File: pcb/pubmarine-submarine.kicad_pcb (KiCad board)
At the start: 2 copper layers, 150.5 x 100 mm, 68 parts, among them J1 GPIO_IN, J10 RPD, J11 Screw_Terminal_01x08, J12 Screw_Terminal_01x08, J13 ADC_HDR, J14 PWM_HDR, J2 GPIO_OUT, J3 FYL, J4 FYR, J5 FPU, J6 FPD, J7 RPU, J8 RYL, J9 RYR, Q1 AO3400A, Q2 AO3400A, Q3 AO3400A, Q4 AO3400A, Q5 AO3400A, Q6 AO3400A, Q7 AO3400A, Q8 AO3400A, U1 A4950E, U2 A4950E, U3 A4950E, U4 A4950E, U5 TLC5947DAP, U6 MCP3008

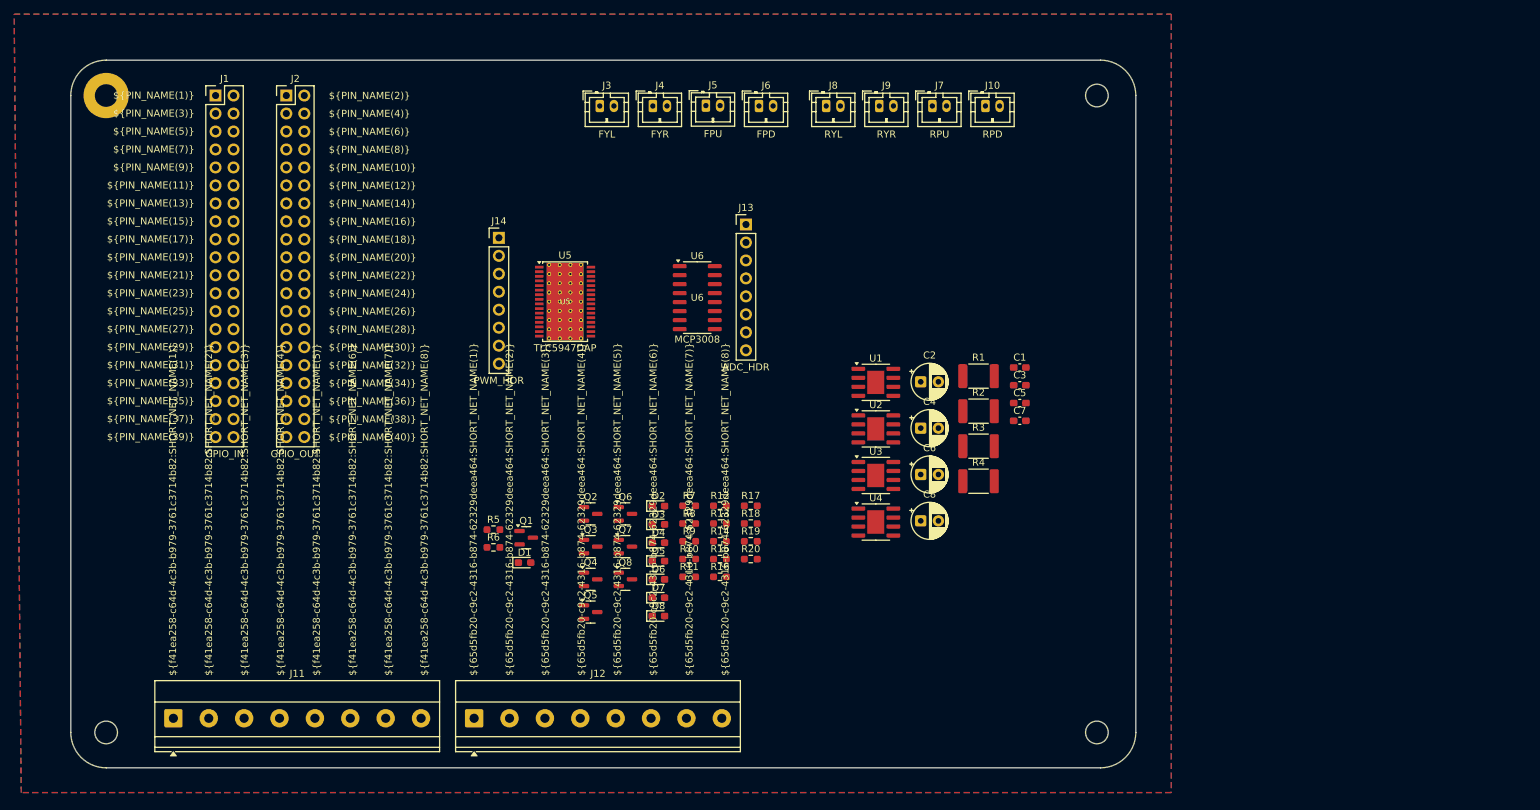
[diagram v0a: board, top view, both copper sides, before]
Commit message: new PCB
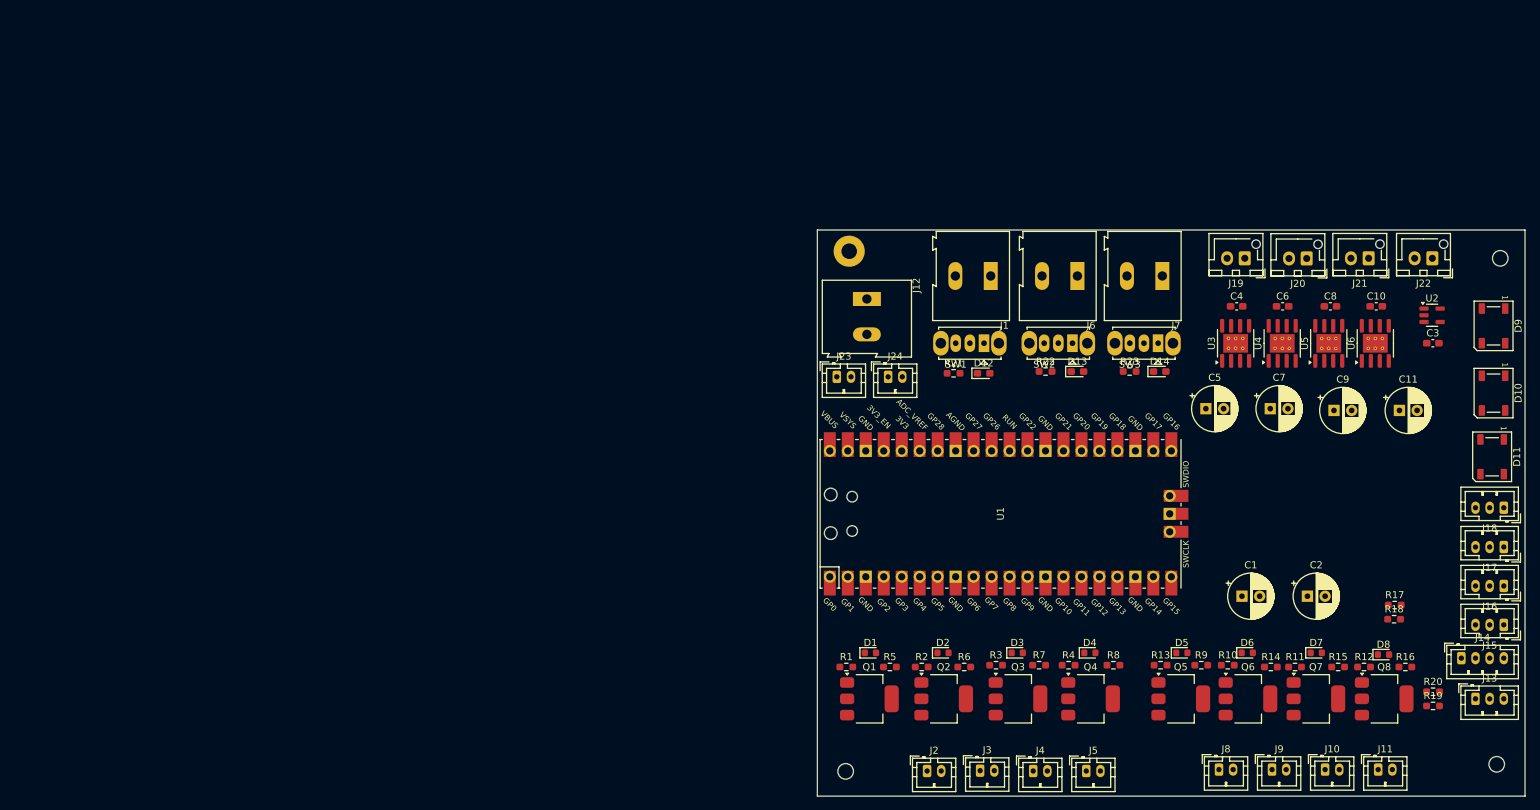
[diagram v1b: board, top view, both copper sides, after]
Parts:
- added C10: 0.22uF, Capacitor_SMD:C_0603_1608Metric_Pad1.08x0.95mm_HandSolder, F.Cu at (254.5, 69.8)
- added C11: 100uF, Capacitor_THT:CP_Radial_D6.3mm_P2.50mm, F.Cu at (257.8, 84.5)
- added C9: 100uF, Capacitor_THT:CP_Radial_D6.3mm_P2.50mm, F.Cu at (248.5, 84.5)
- added D10: WS2812B, LED_SMD:LED_WS2812B_PLCC4_5.0x5.0mm_P3.2mm, F.Cu at (271.1, 82.0)
- added D11: WS2812B, LED_SMD:LED_WS2812B_PLCC4_5.0x5.0mm_P3.2mm, F.Cu at (270.9, 91.0)
- added D12: LED, LED_SMD:LED_0603_1608Metric_Pad1.05x0.95mm_HandSolder, F.Cu at (199.0, 79.2)
- added D13: LED, LED_SMD:LED_0603_1608Metric_Pad1.05x0.95mm_HandSolder, F.Cu at (212.2, 79.0)
- added D14: LED, LED_SMD:LED_0603_1608Metric_Pad1.05x0.95mm_HandSolder, F.Cu at (223.9, 79.0)
- added D9: WS2812B, LED_SMD:LED_WS2812B_PLCC4_5.0x5.0mm_P3.2mm, F.Cu at (271.1, 72.5)
- added J15: Servo1, Connector_JST:JST_PH_B3B-PH-K_1x03_P2.00mm_Vertical, F.Cu at (272.5, 114.8)
- added J16: Servo2, Connector_JST:JST_PH_B3B-PH-K_1x03_P2.00mm_Vertical, F.Cu at (272.5, 109.3)
- added J17: Servo3, Connector_JST:JST_PH_B3B-PH-K_1x03_P2.00mm_Vertical, F.Cu at (272.5, 103.8)
- added J18: Servo4, Connector_JST:JST_PH_B3B-PH-K_1x03_P2.00mm_Vertical, F.Cu at (272.5, 98.2)
- added J19: Conn_01x02, Connector_JST:JST_XH_B2B-XH-AM_1x02_P2.50mm_Vertical, F.Cu at (235.9, 63.0)
- added J20: Conn_01x02, Connector_JST:JST_XH_B2B-XH-AM_1x02_P2.50mm_Vertical, F.Cu at (244.7, 63.0)
- added J21: Conn_01x02, Connector_JST:JST_XH_B2B-XH-AM_1x02_P2.50mm_Vertical, F.Cu at (253.4, 63.0)
- added J22: Conn_01x02, Connector_JST:JST_XH_B2B-XH-AM_1x02_P2.50mm_Vertical, F.Cu at (262.4, 63.0)
- added J23: Conn_01x02, Connector_JST:JST_PH_B2B-PH-K_1x02_P2.00mm_Vertical, F.Cu at (178.2, 79.8)
- added J24: Conn_01x02, Connector_JST:JST_PH_B2B-PH-K_1x02_P2.00mm_Vertical, F.Cu at (185.5, 79.8)
- added R21: 1K, Resistor_SMD:R_0603_1608Metric_Pad0.98x0.95mm_HandSolder, F.Cu at (194.8, 79.2)
- added R22: 330, Resistor_SMD:R_0603_1608Metric_Pad0.98x0.95mm_HandSolder, F.Cu at (207.8, 79.0)
- added R23: 330, Resistor_SMD:R_0603_1608Metric_Pad0.98x0.95mm_HandSolder, F.Cu at (219.6, 79.0)
- added SW1: SW_SPDT, Button_Switch_THT:SW_Slide_SPDT_Straight_CK_OS102011MS2Q, F.Cu at (199.1, 75.0)
- added SW2: SW_SPDT, Button_Switch_THT:SW_Slide_SPDT_Straight_CK_OS102011MS2Q, F.Cu at (211.6, 75.0)
- added SW3: SW_SPDT, Button_Switch_THT:SW_Slide_SPDT_Straight_CK_OS102011MS2Q, F.Cu at (223.7, 75.0)
- C1, C5, C7: value 0.22uF -> 100uF; footprint Capacitor_SMD:C_0603_1608Metric_Pad1.08x0.95mm_HandSolder -> Capacitor_THT:CP_Radial_D6.3mm_P2.50mm
- C2: footprint Capacitor_THT:CP_Radial_D5.0mm_P2.50mm -> Capacitor_THT:CP_Radial_D6.3mm_P2.50mm
- C3: value 0.22uF -> 0.1uF
- C4, C6, C8: value 100uF -> 0.22uF; footprint Capacitor_THT:CP_Radial_D5.0mm_P2.50mm -> Capacitor_SMD:C_0603_1608Metric_Pad1.08x0.95mm_HandSolder
- D1, D2, D3, D4, D5, D6, D7, D8: value D_Schottky -> 1N5822; footprint Diode_SMD:D_0603_1608Metric_Pad1.05x0.95mm_HandSolder -> Diode_SMD:D_0603_1608Metric
- H1: value MountingHole_Pad -> MountingHole; footprint MountingHole:MountingHole_3.2mm_M3_Pad -> MountingHole:MountingHole_2.2mm_M2
- H2, H3: footprint MountingHole:MountingHole_3.2mm_M3 -> MountingHole:MountingHole_2.2mm_M2
- H4: value MountingHole -> MountingHole_Pad; footprint MountingHole:MountingHole_3.2mm_M3 -> MountingHole:MountingHole_2.2mm_M2_Pad
- J1: value GPIO_IN -> Screw_Terminal_01x02; footprint Connector_PinHeader_2.54mm:PinHeader_2x20_P2.54mm_Vertical -> TerminalBlock:TerminalBlock_Altech_AK300-2_P5.00mm
- J10: value RPD -> Conn_01x02
- J11: value Screw_Terminal_01x08 -> Conn_01x02; footprint TerminalBlock_Phoenix:TerminalBlock_Phoenix_MKDS-1,5-8_1x08_P5.00mm_Horizontal -> Connector_JST:JST_PH_B2B-PH-K_1x02_P2.00mm_Vertical
- J12: value Screw_Terminal_01x08 -> Screw_Terminal_01x02; footprint TerminalBlock_Phoenix:TerminalBlock_Phoenix_MKDS-1,5-8_1x08_P5.00mm_Horizontal -> TerminalBlock:TerminalBlock_Altech_AK300-2_P5.00mm
- J13: value ADC_HDR -> Conn_01x03; footprint Connector_PinHeader_2.54mm:PinHeader_1x08_P2.54mm_Vertical -> Connector_JST:JST_PH_B3B-PH-K_1x03_P2.00mm_Vertical
- J14: value PWM_HDR -> Conn_01x04; footprint Connector_PinHeader_2.54mm:PinHeader_1x08_P2.54mm_Vertical -> Connector_JST:JST_PH_B4B-PH-K_1x04_P2.00mm_Vertical
- J2: value GPIO_OUT -> Conn_01x02; footprint Connector_PinHeader_2.54mm:PinHeader_2x20_P2.54mm_Vertical -> Connector_JST:JST_PH_B2B-PH-K_1x02_P2.00mm_Vertical
- J3: value FYL -> Conn_01x02
- J4: value FYR -> Conn_01x02
- J5: value FPU -> Conn_01x02
- J6: value FPD -> Screw_Terminal_01x02; footprint Connector_JST:JST_PH_B2B-PH-K_1x02_P2.00mm_Vertical -> TerminalBlock:TerminalBlock_Altech_AK300-2_P5.00mm
- J7: value RPU -> Screw_Terminal_01x02; footprint Connector_JST:JST_PH_B2B-PH-K_1x02_P2.00mm_Vertical -> TerminalBlock:TerminalBlock_Altech_AK300-2_P5.00mm
- J8: value RYL -> Conn_01x02
- J9: value RYR -> Conn_01x02
- Q1, Q2, Q3, Q4, Q5, Q6, Q7, Q8: value AO3400A -> Q_NMOS_Depletion_DGS; footprint Package_TO_SOT_SMD:SOT-23 -> Package_TO_SOT_SMD:SOT-223-3_TabPin2
- R1, R2, R3, R4: value 1.1Ω -> 470; footprint Resistor_SMD:R_1812_4532Metric_Pad1.30x3.40mm_HandSolder -> Resistor_SMD:R_0603_1608Metric_Pad0.98x0.95mm_HandSolder
- R10, R12: value 100 -> 470
- R11, R9: value 1K -> 470
- R13, R15, R6, R7: value 1K -> 10k
- R14, R16, R5, R8: value 100 -> 10k
- R17: value 1K -> 4.7K
- R18: value 100 -> 4.7K
- R19: value 1K -> 10K
- R20: value 100 -> 20K
- U1: value A4950E -> Pico; footprint Package_SO:SOIC-8-1EP_3.9x4.9mm_P1.27mm_EP2.41x3.3mm -> MCU_RaspberryPi_and_Boards:RPi_Pico_SMD_TH
- U2: value A4950E -> SN74LV1T34DBV; footprint Package_SO:SOIC-8-1EP_3.9x4.9mm_P1.27mm_EP2.41x3.3mm -> Package_TO_SOT_SMD:SOT-23-5
- U3, U4: footprint Package_SO:SOIC-8-1EP_3.9x4.9mm_P1.27mm_EP2.41x3.3mm -> Package_SO:SOIC-8-1EP_3.9x4.9mm_P1.27mm_EP2.62x3.51mm_ThermalVias
- U5: value TLC5947DAP -> A4950E; footprint Package_SO:HTSSOP-32-1EP_6.1x11mm_P0.65mm_EP5.2x11mm_Mask4.11x4.36mm_ThermalVias -> Package_SO:SOIC-8-1EP_3.9x4.9mm_P1.27mm_EP2.62x3.51mm_ThermalVias
- U6: value MCP3008 -> A4950E; footprint Package_SO:SOIC-16_3.9x9.9mm_P1.27mm -> Package_SO:SOIC-8-1EP_3.9x4.9mm_P1.27mm_EP2.62x3.51mm_ThermalVias
- moved H1 198.3 mm to (272.0, 63.0)
- moved J11 170.4 mm to (254.8, 135.2)
- moved J14 148.4 mm to (266.5, 119.5)
- moved J2 131.6 mm to (191.0, 135.4)
- moved J13 123.0 mm to (268.5, 125.2)
- moved J1 112.5 mm to (200.0, 65.5), turned to 180 degrees
- moved H2 110.1 mm to (271.5, 134.5)
- moved J8 109.0 mm to (232.2, 135.2)
- moved J9 109.0 mm to (239.8, 135.2)
- moved Q8 108.6 mm to (255.6, 125.2)
- moved J5 108.3 mm to (213.5, 135.4)
- moved J4 108.3 mm to (206.0, 135.4)
- moved J3 108.2 mm to (198.5, 135.4)
- moved U5 108.1 mm to (247.8, 75.0), turned to 90 degrees
- moved J10 105.3 mm to (247.2, 135.2)
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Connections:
- C1 pad 1: +12VA -> +5VP
- C1 pad 2: GNDA -> GND
- C2 pad 1: +12VA -> +5VP
- C2 pad 2: GNDA -> GND
- C3 pad 1: +12VA -> +5VL
- C3 pad 2: GNDA -> GND
- C4 pad 1: +12VA -> +12V
- C4 pad 2: GNDA -> GND
- C5 pad 1: +12VA -> +12V
- C5 pad 2: GNDA -> GND
- C6 pad 1: +12VA -> +12V
- C6 pad 2: GNDA -> GND
- C7 pad 1: +12VA -> +12V
- C7 pad 2: GNDA -> GND
- C8 pad 1: +12VA -> +12V
- C8 pad 2: GNDA -> GND
- D1 pad 1: +12VA -> +5VP
- D1 pad 2: FYL- -> /FU-
- D2 pad 1: +12VA -> +5VP
- D2 pad 2: FYR- -> /FD-
- D3 pad 1: +12VA -> +5VP
- D3 pad 2: FPU- -> /FL-
- D4 pad 1: +12VA -> +5VP
- D4 pad 2: FPD- -> /FR-
- D5 pad 1: +12VA -> +5VP
- D5 pad 2: RYL- -> /RU-
- D6 pad 1: +12VA -> +5VP
- D6 pad 2: RYR- -> /RD-
- D7 pad 1: +12VA -> +5VP
- D7 pad 2: RPU- -> /RL-
- D8 pad 1: +12VA -> +5VP
- D8 pad 2: RPD- -> /RR-
- J1 pad 1: unconnected-(J1-3V3-Pad1) -> Net-(J1-Pin_1)
- J1 pad 2: +5VD -> GND
- J10 pad 1: +12VA -> +5VP
- J10 pad 2: RPD- -> /RL-
- J11 pad 1: +12VA -> +5VP
- J11 pad 2: GNDA -> /RR-
- J12 pad 1: X+ -> +5VL
- J12 pad 2: X- -> GND
- J13 pad 1: CH0 -> GND
- J13 pad 2: CH1 -> +5VL
- J13 pad 3: CH2 -> Net-(J13-Pin_3)
- J14 pad 1: PWM16 -> GND
- J14 pad 2: PWM17 -> +5VL
- J14 pad 3: PWM18 -> SDA
- J14 pad 4: PWM19 -> SCL
- J2 pad 1: unconnected-(J2-3V3-Pad1) -> +5VP
- J2 pad 2: +5VD -> /FU-
- J3 pad 1: +12VA -> +5VP
- J3 pad 2: FYL- -> /FD-
- J4 pad 1: +12VA -> +5VP
- J4 pad 2: FYR- -> /FL-
- J5 pad 1: +12VA -> +5VP
- J5 pad 2: FPU- -> /FR-
- J6 pad 1: +12VA -> Net-(J6-Pin_1)
- J6 pad 2: FPD- -> GND
- J7 pad 1: +12VA -> Net-(J7-Pin_1)
- J7 pad 2: RPU- -> GND
- J8 pad 1: +12VA -> +5VP
- J8 pad 2: RYL- -> /RU-
- J9 pad 1: +12VA -> +5VP
- J9 pad 2: RYR- -> /RD-
- Q1 pad 1: Net-(Q1-G) -> /FU-
- Q1 pad 2: GND -> Net-(Q1-G)
- Q1 pad 3: FYL- -> GND
- Q2 pad 1: Net-(Q2-G) -> /FD-
- Q2 pad 2: GND -> Net-(Q2-G)
- Q2 pad 3: FYR- -> GND
- Q3 pad 1: Net-(Q3-G) -> /FL-
- Q3 pad 2: GND -> Net-(Q3-G)
- Q3 pad 3: FPU- -> GND
- Q4 pad 1: Net-(Q4-G) -> /FR-
- Q4 pad 2: GND -> Net-(Q4-G)
- Q4 pad 3: FPD- -> GND
- Q5 pad 1: Net-(Q5-G) -> /RU-
- Q5 pad 2: GND -> Net-(Q5-G)
- Q5 pad 3: RYL- -> GND
- Q6 pad 1: Net-(Q6-G) -> /RD-
- Q6 pad 2: GND -> Net-(Q6-G)
- Q6 pad 3: RYR- -> GND
- Q7 pad 1: Net-(Q7-G) -> /RL-
- Q7 pad 2: GND -> Net-(Q7-G)
- Q7 pad 3: RPU- -> GND
- Q8 pad 1: Net-(Q8-G) -> /RR-
- Q8 pad 2: GND -> Net-(Q8-G)
- Q8 pad 3: RPD- -> GND
- R1 pad 1: Net-(U1-LSS) -> FU
- R1 pad 2: GNDA -> Net-(Q1-G)
- R10 pad 1: PWM10 -> RD
- R10 pad 2: Net-(Q3-G) -> Net-(Q6-G)
- R11 pad 1: PWM11 -> RL
- R11 pad 2: GND -> Net-(Q7-G)
- R12 pad 1: PWM11 -> RR
- R12 pad 2: Net-(Q4-G) -> Net-(Q8-G)
- R13 pad 1: PWM12 -> Net-(Q5-G)
- R14 pad 1: PWM12 -> Net-(Q6-G)
- R14 pad 2: Net-(Q5-G) -> GND
- R15 pad 1: PWM13 -> Net-(Q7-G)
- R16 pad 1: PWM13 -> Net-(Q8-G)
- R16 pad 2: Net-(Q6-G) -> GND
- R17 pad 1: PWM14 -> SDA
- R17 pad 2: GND -> +5VL
- R18 pad 1: PWM14 -> SCL
- R18 pad 2: Net-(Q7-G) -> +5VL
- R19 pad 1: PWM15 -> Net-(J13-Pin_3)
- R19 pad 2: GND -> SENS1
- R2 pad 1: Net-(U2-LSS) -> FD
- R2 pad 2: GNDA -> Net-(Q2-G)
- R20 pad 1: PWM15 -> SENS1
- R20 pad 2: Net-(Q8-G) -> GND
- R3 pad 1: Net-(U3-LSS) -> FL
- R3 pad 2: GNDA -> Net-(Q3-G)
- R4 pad 1: Net-(U4-LSS) -> FR
- R4 pad 2: GNDA -> Net-(Q4-G)
- R5 pad 1: PWM8 -> Net-(Q1-G)
- R5 pad 2: Net-(Q1-G) -> GND
- R6 pad 1: PWM8 -> Net-(Q2-G)
- R7 pad 1: PWM9 -> Net-(Q3-G)
- R8 pad 1: PWM9 -> Net-(Q4-G)
- R8 pad 2: Net-(Q2-G) -> GND
- R9 pad 1: PWM10 -> RU
- R9 pad 2: GND -> Net-(Q5-G)
- U1 pad 1: GNDA -> LED_DATA
- U1 pad 2: unconnected-(U1-IN2-Pad2) -> IN_W2
- U1 pad 3: unconnected-(U1-IN1-Pad3) -> GND
- U1 pad 4: +3V3 -> SDA
- U1 pad 5: +12VA -> SCL
- U1 pad 6: X+ -> FU
- U1 pad 7: Net-(U1-LSS) -> FD
- U1 pad 8: X- -> GND
- U1 pad 9: GNDA -> FL
- U2 pad 1: GNDA -> unconnected-(U2-NC-Pad1)
- U2 pad 2: unconnected-(U2-IN2-Pad2) -> LED_DATA
- U2 pad 3: unconnected-(U2-IN1-Pad3) -> GND
- U2 pad 4: +3V3 -> Net-(D9-DIN)
- U2 pad 5: +12VA -> +5VL
- U3 pad 1: GNDA -> GND
- U3 pad 2: unconnected-(U3-IN2-Pad2) -> IN_X2
- U3 pad 3: unconnected-(U3-IN1-Pad3) -> IN_X1
- U3 pad 4: +3V3 -> +3.3V
- U3 pad 5: +12VA -> +12V
- U3 pad 6: X+ -> /X+
- U3 pad 7: Net-(U3-LSS) -> unconnected-(U3-LSS-Pad7)
- U3 pad 8: X- -> /X-
- U3 pad 9: GNDA -> GND
- U4 pad 1: GNDA -> GND
- U4 pad 2: unconnected-(U4-IN2-Pad2) -> IN_Y2
- U4 pad 3: unconnected-(U4-IN1-Pad3) -> IN_Y1
- U4 pad 4: +3V3 -> +3.3V
- U4 pad 5: +12VA -> +12V
- U4 pad 6: X+ -> /Y+
- U4 pad 7: Net-(U4-LSS) -> unconnected-(U4-LSS-Pad7)
- U4 pad 8: X- -> /Y-
- U4 pad 9: GNDA -> GND
- U5 pad 2: unconnected-(U5-BLANK-Pad2) -> IN_Z2
- U5 pad 3: unconnected-(U5-SCLK-Pad3) -> IN_Z1
- U5 pad 4: unconnected-(U5-SIN-Pad4) -> +3.3V
- U5 pad 5: PWM0 -> +12V
- U5 pad 6: PWM1 -> /Z+
- U5 pad 7: PWM2 -> unconnected-(U5-LSS-Pad7)
- U5 pad 8: PWM3 -> /Z-
- U5 pad 9: PWM4 -> GND
- U6 pad 1: CH0 -> GND
- U6 pad 2: CH1 -> IN_W2
- U6 pad 3: CH2 -> IN_W1
- U6 pad 4: CH3 -> +3.3V
- U6 pad 5: CH4 -> +12V
- U6 pad 6: CH5 -> /W+
- U6 pad 7: CH6 -> unconnected-(U6-LSS-Pad7)
- U6 pad 8: CH7 -> /W-
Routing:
- removed copper zone on B.Cu, net GND
- removed copper zone on F.Cu, net GND
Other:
- board size 150.5 x 100 mm -> 100 x 80 mm
- board text removed: "${65d5fb20-c9c2-4316-b874-62329deea464:SHORT_NET_NAME(1)}"
- board text removed: "${65d5fb20-c9c2-4316-b874-62329deea464:SHORT_NET_NAME(2)}"
- board text removed: "${65d5fb20-c9c2-4316-b874-62329deea464:SHORT_NET_NAME(3)}"
- board text removed: "${65d5fb20-c9c2-4316-b874-62329deea464:SHORT_NET_NAME(4)}"
- board text removed: "${65d5fb20-c9c2-4316-b874-62329deea464:SHORT_NET_NAME(5)}"
- board text removed: "${65d5fb20-c9c2-4316-b874-62329deea464:SHORT_NET_NAME(6)}"
- board text removed: "${65d5fb20-c9c2-4316-b874-62329deea464:SHORT_NET_NAME(7)}"
- board text removed: "${65d5fb20-c9c2-4316-b874-62329deea464:SHORT_NET_NAME(8)}"
- board text removed: "${f41ea258-c64d-4c3b-b979-3761c3714b82:SHORT_NET_NAME(1)}"
- board text removed: "${f41ea258-c64d-4c3b-b979-3761c3714b82:SHORT_NET_NAME(2)}"
- board text removed: "${f41ea258-c64d-4c3b-b979-3761c3714b82:SHORT_NET_NAME(3)}"
- board text removed: "${f41ea258-c64d-4c3b-b979-3761c3714b82:SHORT_NET_NAME(4)}"
- board text removed: "${f41ea258-c64d-4c3b-b979-3761c3714b82:SHORT_NET_NAME(5)}"
- board text removed: "${f41ea258-c64d-4c3b-b979-3761c3714b82:SHORT_NET_NAME(6)}"
- board text removed: "${f41ea258-c64d-4c3b-b979-3761c3714b82:SHORT_NET_NAME(7)}"
- board text removed: "${f41ea258-c64d-4c3b-b979-3761c3714b82:SHORT_NET_NAME(8)}"
